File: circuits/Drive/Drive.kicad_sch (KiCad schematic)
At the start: 25 parts, among them J1 Conn_01x14_Pin, Q15 BSS138, Q16 BSS138, SW1 SW_SPST, SW5 SW_SPST, U2 STM32F446RETx, Y2 16MHz

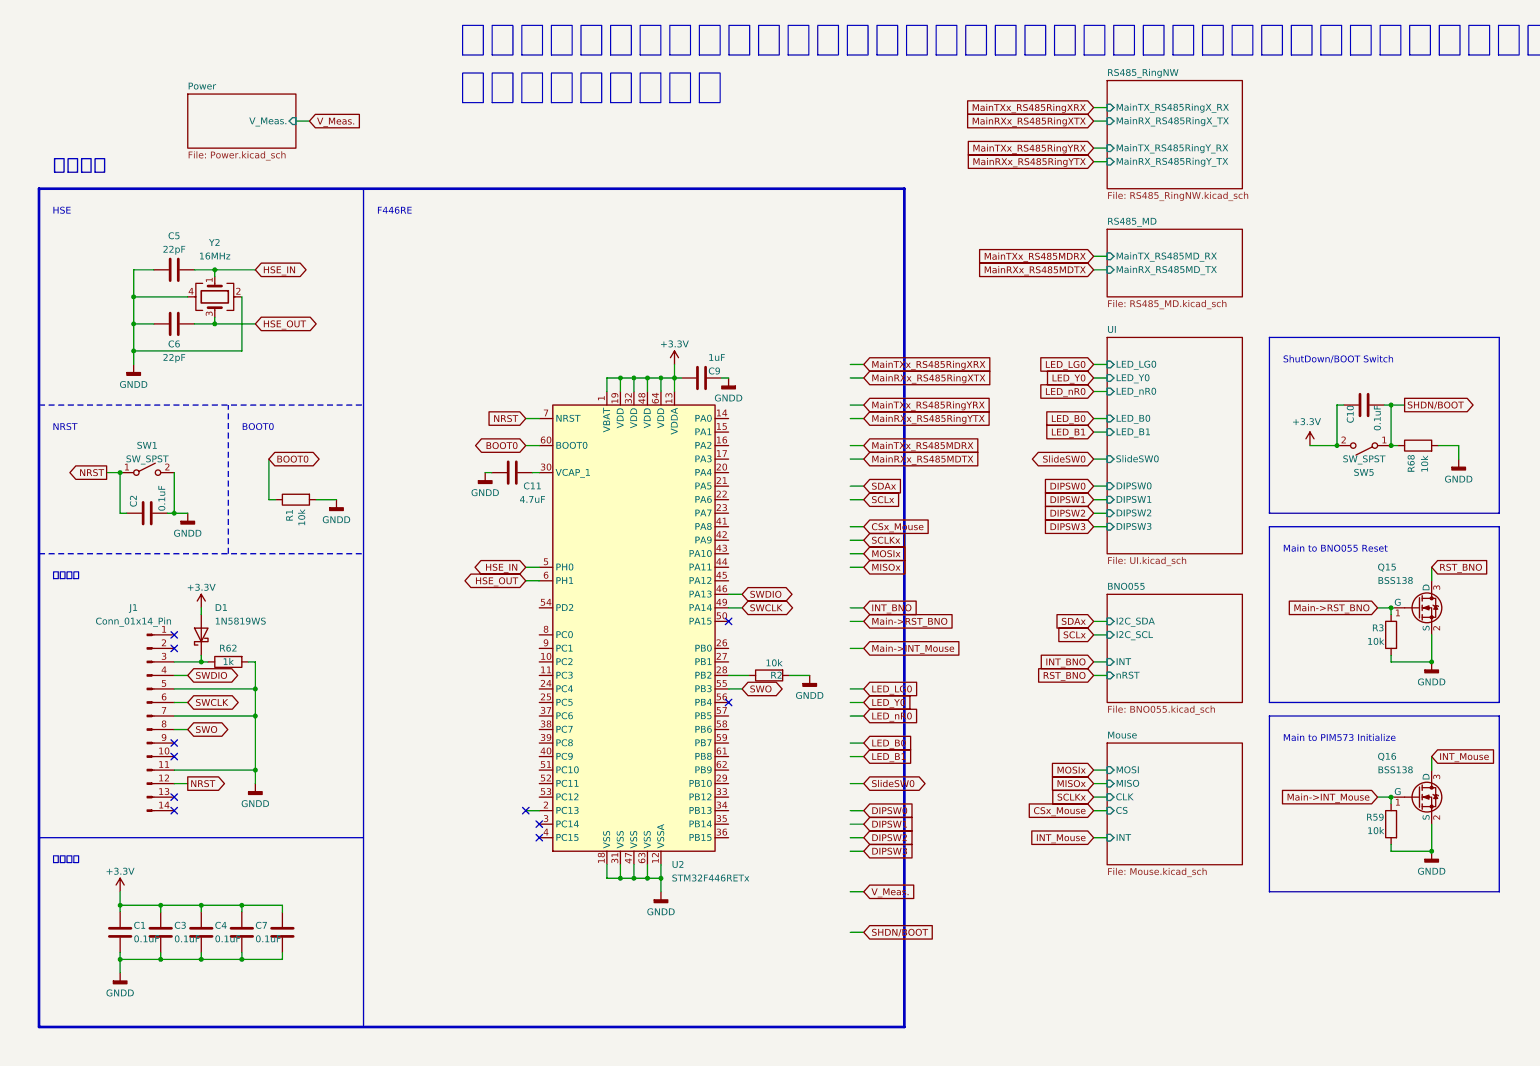
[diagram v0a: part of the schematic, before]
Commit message: 更新
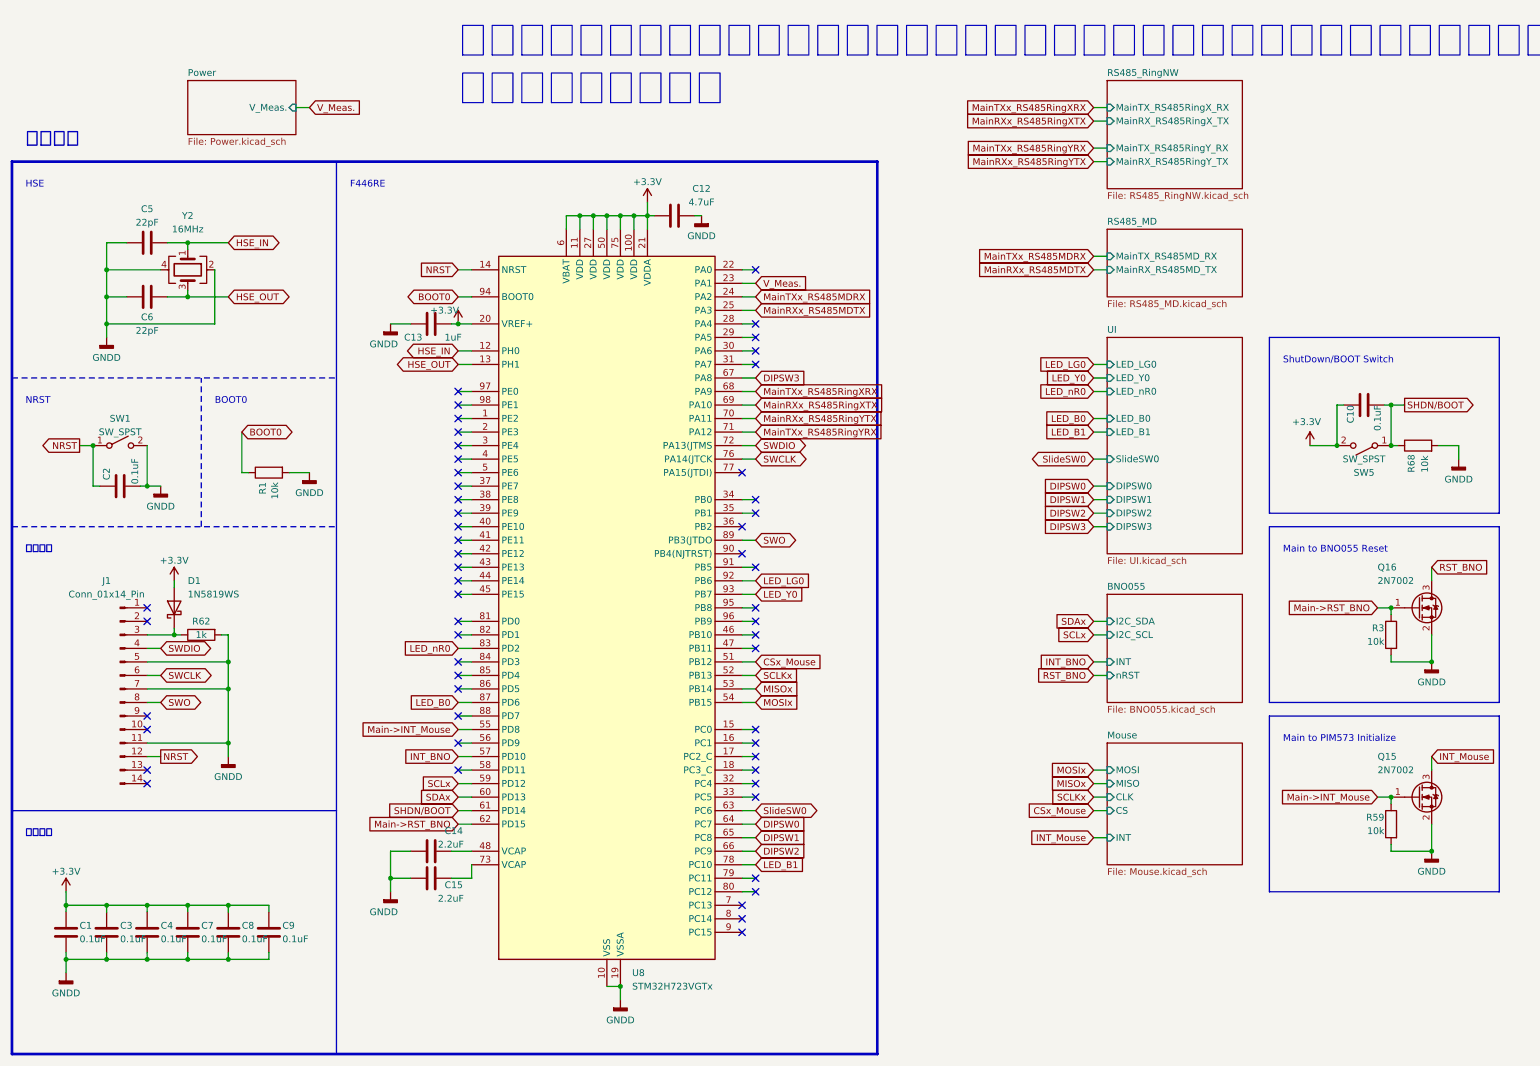
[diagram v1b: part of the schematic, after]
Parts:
- removed C11: 4.7uF, Capacitor_SMD:C_0603_1608Metric, symbol Device:C
- removed Q15, Q16: BSS138, Package_TO_SOT_SMD:SOT-23, symbol Device:Q_NMOS_GSD
- removed R2: 10k, Resistor_SMD:R_0402_1005Metric, symbol Device:R
- removed U2: STM32F446RETx, Package_QFP:LQFP-64_10x10mm_P0.5mm, symbol MCU_ST_STM32F4:STM32F446RETx
- added C12: 4.7uF, Capacitor_SMD:C_0603_1608Metric, symbol Device:C
- added C13: 1uF, Capacitor_SMD:C_0402_1005Metric, symbol Device:C
- added C14, C15: 2.2uF, Capacitor_SMD:C_0402_1005Metric, symbol Device:C
- added Q15, Q16: 2N7002, Package_TO_SOT_SMD:SOT-23, symbol Transistor_FET:2N7002
- added U8: STM32H723VGTx, Package_QFP:LQFP-100_14x14mm_P0.5mm, symbol MCU_ST_STM32H7:STM32H723VGTx
- C9: value 1uF -> 0.1uF
- SW5: footprint (none) -> Button_Switch_THT:SW_PUSH_1P1T_6x3.5mm_H4.3_APEM_MJTP1243
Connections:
- net +3.3V: now also C9.1, C12.1, C13.1, U8.100 (VDD), U8.11 (VDD), U8.20 (VREF+), U8.21 (VDDA), U8.27 (VDD), U8.50 (VDD), U8.6 (VBAT), U8.75 (VDD); no longer C9.2
- net BOOT0: now also U8.94 (BOOT0)
- net CSx_Mouse: now also U8.51 (PB12)
- net DIPSW0: now also U8.64 (PC7)
- net DIPSW1: now also U8.65 (PC8)
- net DIPSW2: now also U8.66 (PC9)
- net DIPSW3: now also U8.67 (PA8)
- net GNDD: now also C9.2, C12.2, C13.2, C14.2, C15.2, Q15.2 (S), Q16.2 (S), U8.10 (VSS), U8.19 (VSSA), U8.26 (VSS), U8.49 (VSS), U8.74 (VSS), U8.99 (VSS); no longer C9.1
- net HSE_IN: now also U8.12 (PH0)
- net HSE_OUT: now also U8.13 (PH1)
- net INT_BNO: now also U8.57 (PD10)
- net INT_Mouse: now also Q15.3 (D)
- net LED_B0: now also U8.87 (PD6)
- net LED_B1: now also U8.78 (PC10)
- net LED_LG0: now also U8.92 (PB6)
- net LED_Y0: now also U8.93 (PB7)
- net LED_nR0: now also U8.83 (PD2)
- net MISOx: now also U8.53 (PB14)
- net MOSIx: now also U8.54 (PB15)
- net Main->INT_Mouse: now also Q15.1 (G), U8.55 (PD8)
- net Main->RST_BNO: now also Q16.1 (G), U8.62 (PD15)
- net MainRXx_RS485MDTX: now also U8.25 (PA3)
- net MainRXx_RS485RingXTX: now also U8.69 (PA10)
- net MainRXx_RS485RingYTX: now also U8.70 (PA11)
- net MainTXx_RS485MDRX: now also U8.24 (PA2)
- net MainTXx_RS485RingXRX: now also U8.68 (PA9)
- net MainTXx_RS485RingYRX: now also U8.71 (PA12)
- net NRST: now also U8.14 (NRST)
- net RST_BNO: now also Q16.3 (D)
- net SCLKx: now also U8.52 (PB13)
- net SCLx: now also U8.59 (PD12)
- net SDAx: now also U8.60 (PD13)
- net SHDN/BOOT: now also U8.61 (PD14)
- net SWCLK: now also U8.76 (PA14(JTCK)
- net SWDIO: now also U8.72 (PA13(JTMS)
- net SWO: now also U8.89 (PB3(JTDO)
- net SlideSW0: now also U8.63 (PC6)
- net V_Meas.: now also U8.23 (PA1)
- new net: C14.1, U8.48 (VCAP)
- new net: C15.1, U8.73 (VCAP)
- no-connect marks 11 -> 56
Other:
- moved on the sheet: C1, C2, C3, C4, C5, C6, C7, D1, J1, R1, R62, SW1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

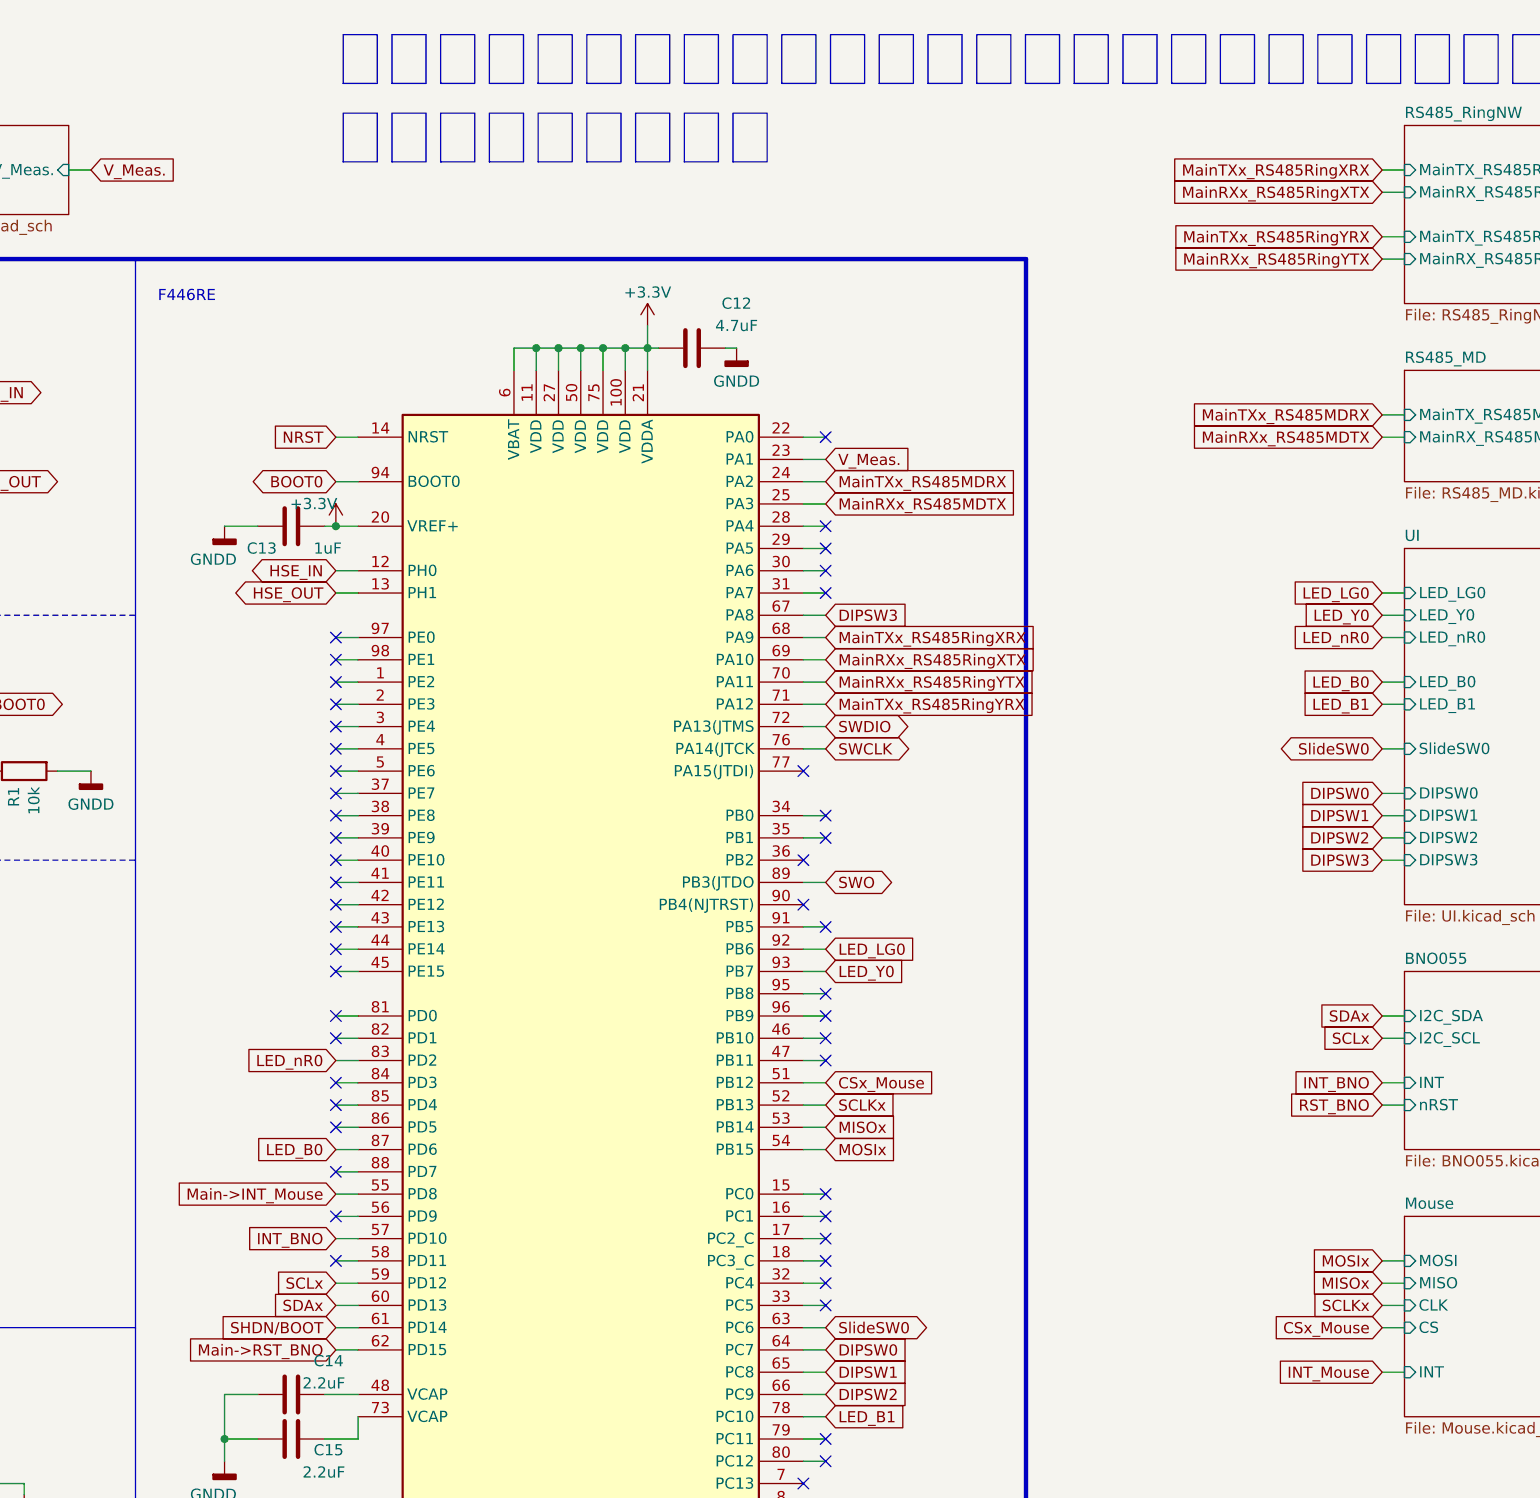
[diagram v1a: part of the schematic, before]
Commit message: raspi基板回路図
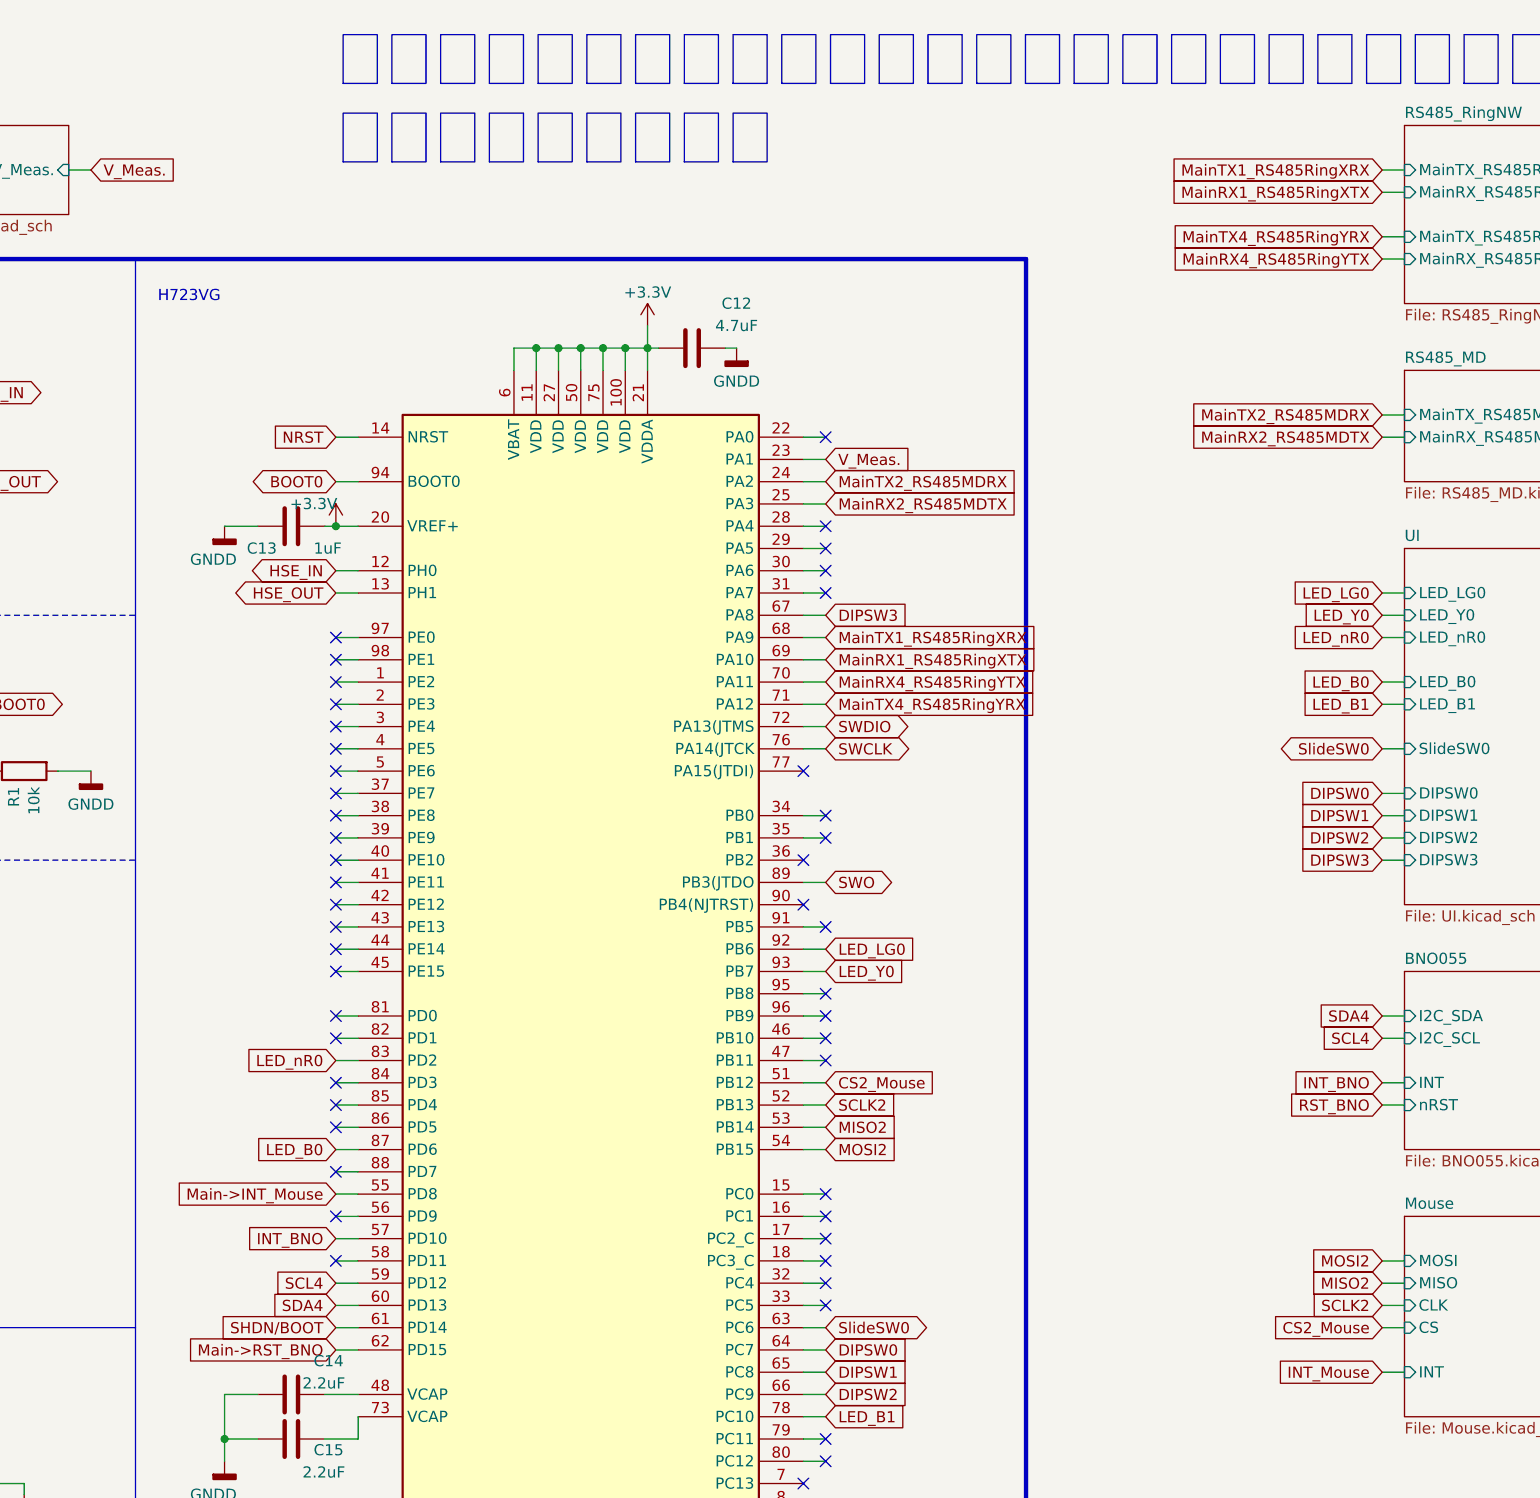
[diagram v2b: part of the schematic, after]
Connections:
- net CSx_Mouse renamed CS2_Mouse
- net MISOx renamed MISO2
- net MOSIx renamed MOSI2
- net MainRXx_RS485MDTX renamed MainRX2_RS485MDTX
- net MainRXx_RS485RingXTX renamed MainRX1_RS485RingXTX
- net MainRXx_RS485RingYTX renamed MainRX4_RS485RingYTX
- net MainTXx_RS485MDRX renamed MainTX2_RS485MDRX
- net MainTXx_RS485RingXRX renamed MainTX1_RS485RingXRX
- net MainTXx_RS485RingYRX renamed MainTX4_RS485RingYRX
- net SCLKx renamed SCLK2
- net SCLx renamed SCL4
- net SDAx renamed SDA4
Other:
- note added: "H723VG"
- note removed: "F446RE"
